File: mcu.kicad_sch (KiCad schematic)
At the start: 20 parts, among them U1 ESP32-S2FN4R2, Y1 ECX-1637B2

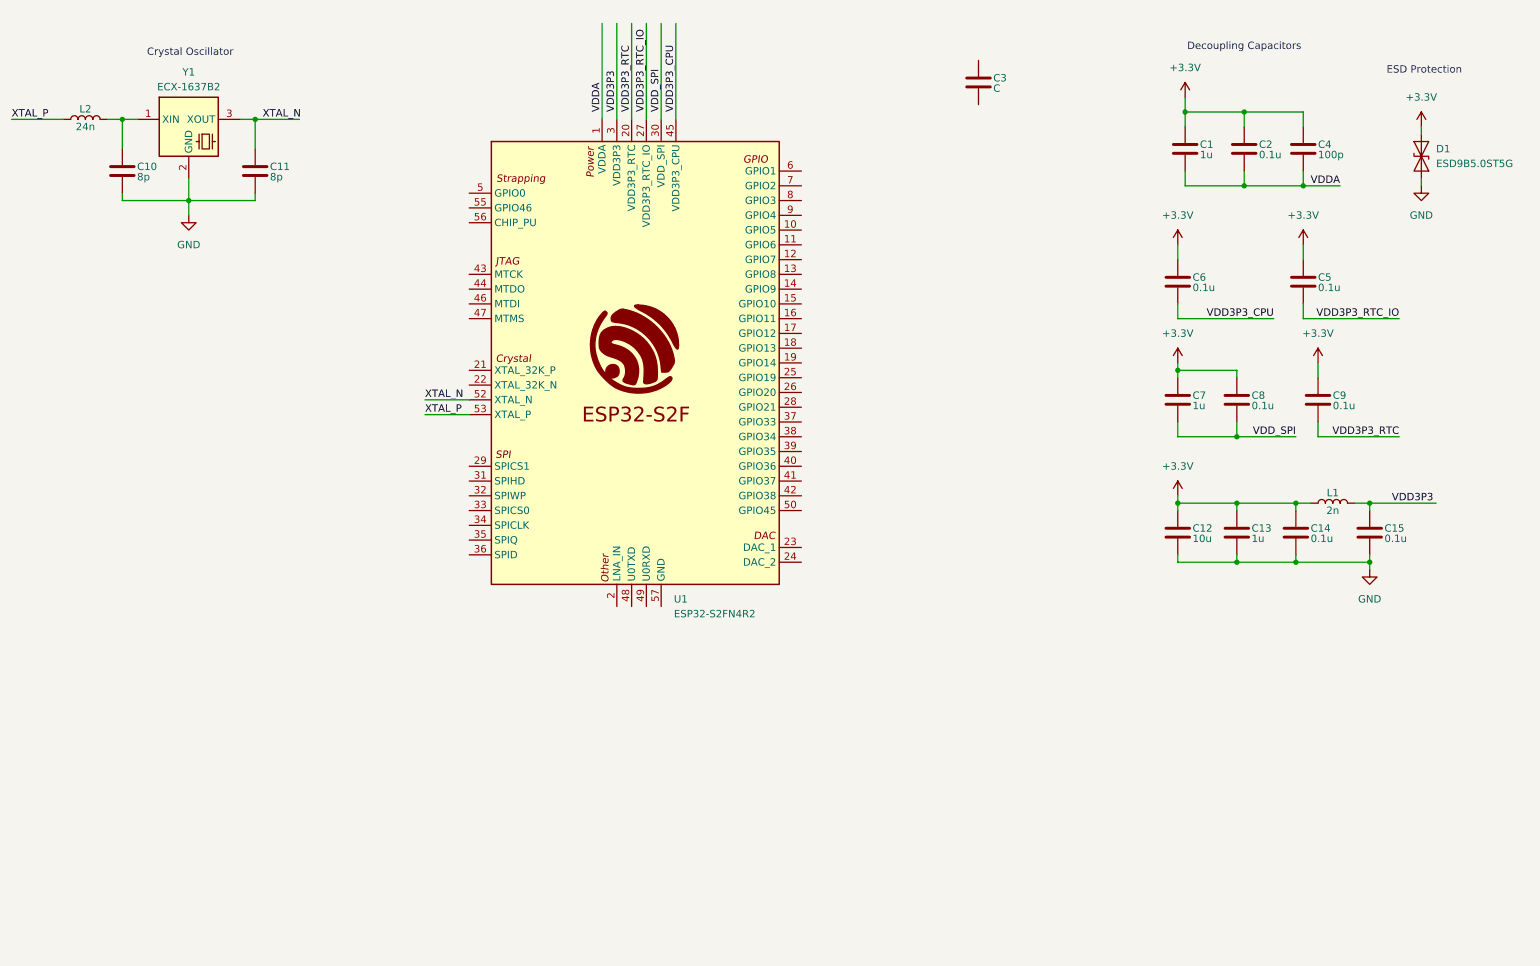
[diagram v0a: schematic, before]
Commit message: Add files via upload
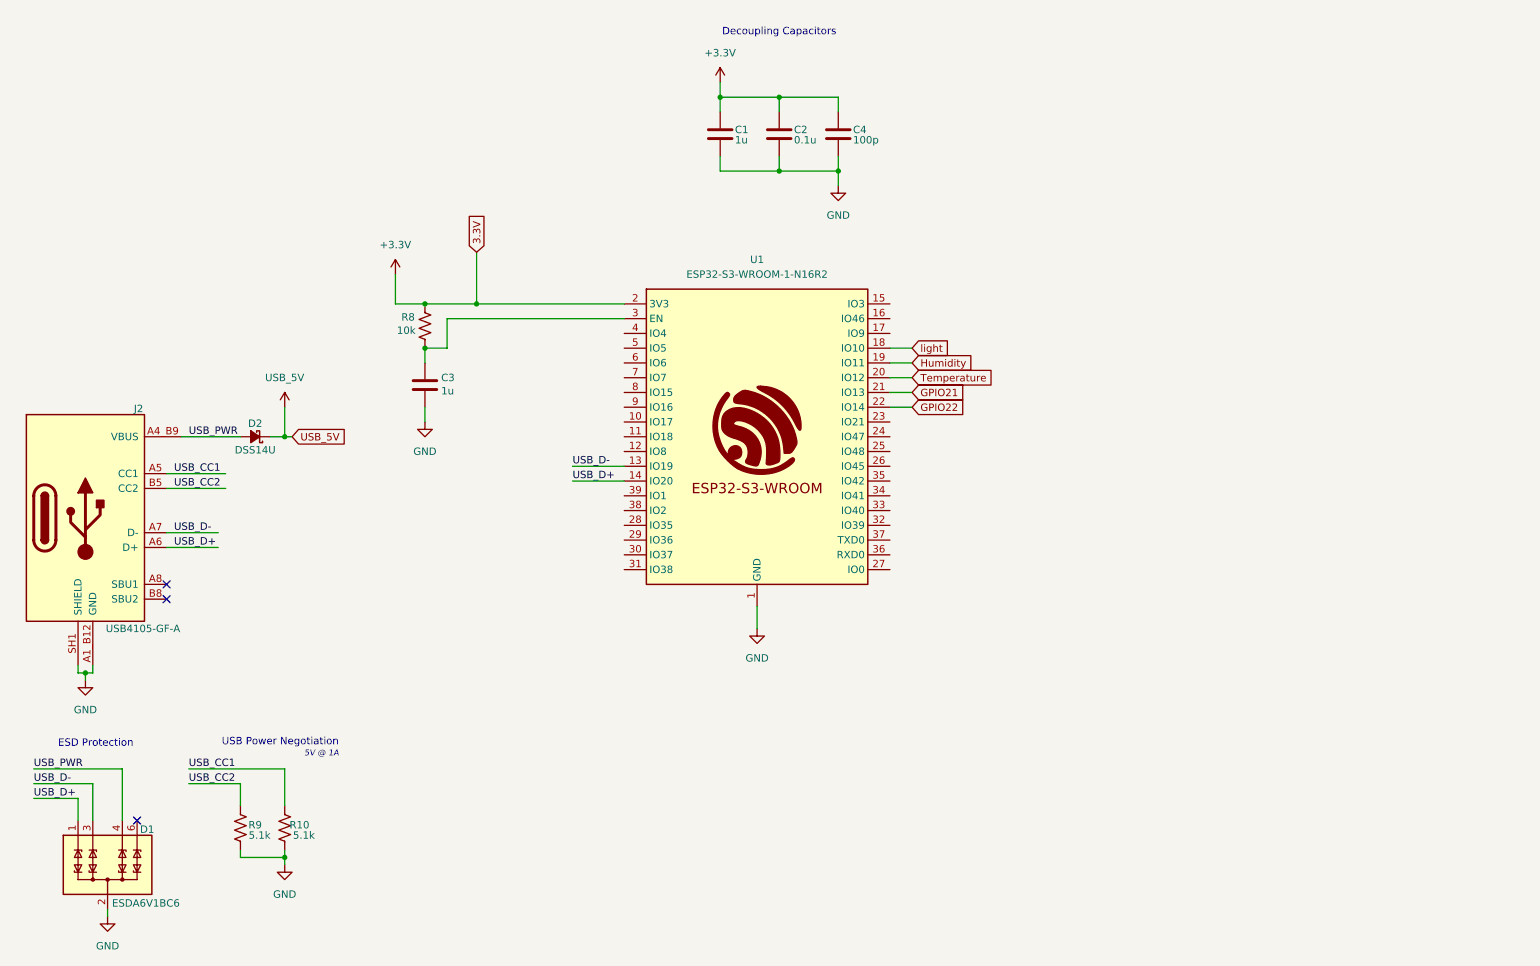
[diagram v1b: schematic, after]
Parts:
- removed C10, C11: 8p, Capacitor_SMD:C_0805_2012Metric_Pad1.18x1.45mm_HandSolder, symbol Device:C
- removed C12: 10u, Capacitor_SMD:C_0805_2012Metric_Pad1.18x1.45mm_HandSolder, symbol Device:C
- removed C13, C7: 1u, Capacitor_SMD:C_0805_2012Metric_Pad1.18x1.45mm_HandSolder, symbol Device:C
- removed C14, C15, C5, C6, C8, C9: 0.1u, Capacitor_SMD:C_0805_2012Metric_Pad1.18x1.45mm_HandSolder, symbol Device:C
- removed D1: ESD9B5.0ST5G, Diode_SMD:D_SOD-923, symbol Diode:ESD9B5.0ST5G
- removed L1: 2n, symbol Device:L
- removed L2: 24n, symbol Device:L
- removed U1: ESP32-S2FN4R2, symbol AA_MCUs:ESP32-S2FN4R2
- removed Y1: ECX-1637B2, symbol AA_Crystals:ECX-1637B2
- added D1: ESDA6V1BC6, Package_TO_SOT_SMD:SOT-23-6, symbol Power_Protection:ESDA6V1BC6
- added D2: DSS14U, AA_Diodes:SOD-123FL, symbol Device:D_Schottky_Small_Filled
- added J2: USB4105-GF-A, AA_Connectors:GCT_USB4105-GF-A, symbol AA_Connectors:USB4105-GF-A
- added R10, R9: 5.1k, Resistor_SMD:R_0805_2012Metric, symbol Device:R_US
- added R8: 10k, symbol Device:R_US
- added U1: ESP32-S3-WROOM-1-N16R2, AA_MCUs:ESP32S3WROOM1N16R2, symbol AA_MCUs:ESP32-S3-WROOM-1-N16R2
- C3: value C -> 1u; footprint Capacitor_SMD:C_0805_2012Metric_Pad1.18x1.45mm_HandSolder -> (none)
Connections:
- net VDDA is gone; now on net EPAD: C1.2, C2.2, C4.2
- net +3.3V: now also R8.1, U1.2 (3V3)
- net at C3.1: now also R8.2, U1.3 (EN)
- net EPAD: now reaches C3.2
- net EPAD: now also D1.2 (COM), D1.5 (COM), J2.A1_B12 (GND), J2.B1_A12 (GND), J2.SH1 (SHIELD), J2.SH2 (SHIELD), J2.SH3 (SHIELD), J2.SH4 (SHIELD), R10.1, R9.1, U1.1 (GND), U1.40 (GND), U1.41 (EPAD)
- new net GPIO21: U1.21 (IO13)
- new net GPIO22: U1.22 (IO14)
- new net Humidity: U1.19 (IO11)
- new net Temperature: U1.20 (IO12)
- new net USB_5V: D2.1 (K)
- new net USB_CC1: J2.A5 (CC1), R10.2
- new net USB_CC2: J2.B5 (CC2), R9.2
- new net USB_D+: D1.1 (TVS1), J2.A6 (D+), J2.B6 (D+), U1.14 (IO20)
- new net USB_D-: D1.3 (TVS2), J2.A7 (D-), J2.B7 (D-), U1.13 (IO19)
- new net VBUS: D1.4 (TVS3), D2.2 (A), J2.A4_B9 (VBUS), J2.B4_A9 (VBUS)
- new net light: U1.18 (IO10)
- no-connect marks 0 -> 3
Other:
- note added: "5V @ 1A"
- note added: "USB Power Negotiation"
- note removed: "Crystal Oscillator"
- moved on the sheet: C1, C2, C4
